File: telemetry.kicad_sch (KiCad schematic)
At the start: 72 parts, among them J1 Conn_01x03, J10 DT13-2P, J11 Conn_01x03, J12 Conn_01x03, J13 Conn_01x03, J14 Conn_01x06, J15 Conn_01x03, J16 Conn_01x03, J17 Conn_01x03, J18 Conn_01x03, J19 Conn_01x03, J2 DT13-2P, J20 DT13-2P, J21 DT13-2P, J22 Conn_01x03, J3 Conn_01x06, J4 Conn_01x06, J5 Conn_01x06, J6 Conn_01x06, J7 Conn_01x06, J8 Conn_01x06, J9 Micro_SD_Card, Q1 BS170F, Q2 BS170F, U2 Waveshare ESP32-S3 Devboard, U3 TLV76133DCY, U4 DS1307+, U5 R-78C5.0-1.0, U6 MCP2551-I-P, Y2 ABS07-32.768KHZ-T

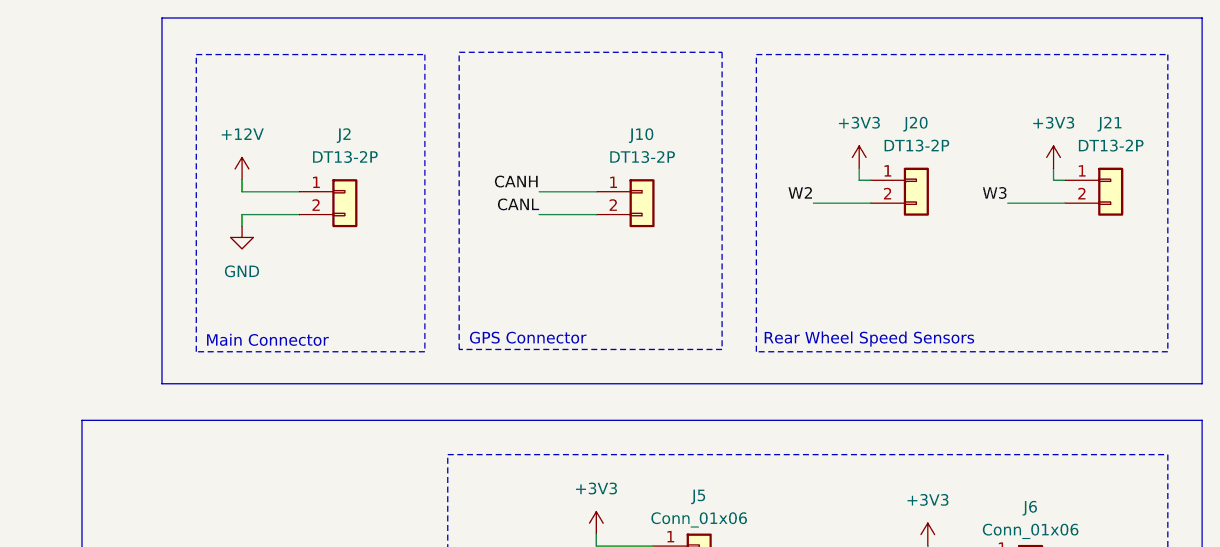
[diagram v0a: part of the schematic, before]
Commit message: Slim board
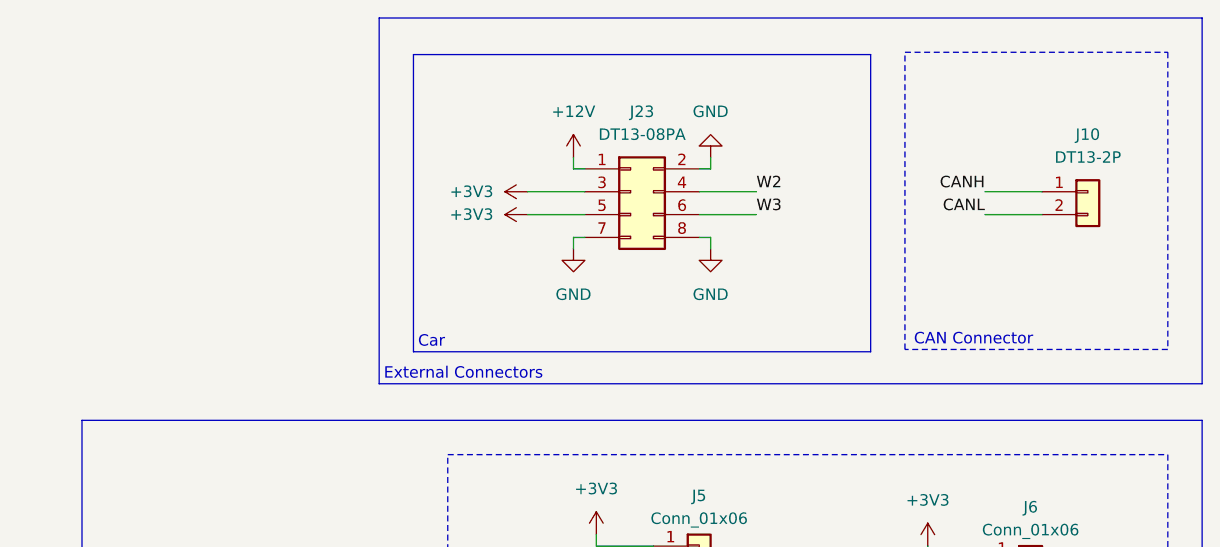
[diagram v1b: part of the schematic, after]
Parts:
- removed J2, J20, J21: DT13-2P, Connector_DT:TE_DT13-2P, symbol Connector_Generic:Conn_01x02
- added J23: DT13-08PA, Connector_DT:TE_DT13-08PA, symbol Connector_Generic:Conn_02x04_Odd_Even
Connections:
- net +12V: now also J23.1 (Pin_1)
- net +3V3: now also J23.3 (Pin_3), J23.5 (Pin_5)
- net GND: now also J23.2 (Pin_2), J23.7 (Pin_7), J23.8 (Pin_8)
- net W2: now also J23.4 (Pin_4)
- net W3: now also J23.6 (Pin_6)
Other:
- note added: "CAN Connector"
- note added: "Car"
- note removed: "GPS Connector"
- note removed: "Main Connector"
- note removed: "Rear Wheel Speed Sensors"
- moved on the sheet: J10
